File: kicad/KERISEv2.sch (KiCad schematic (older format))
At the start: 11 parts, among them SW1 RESET, U1 STM32F405RGTx

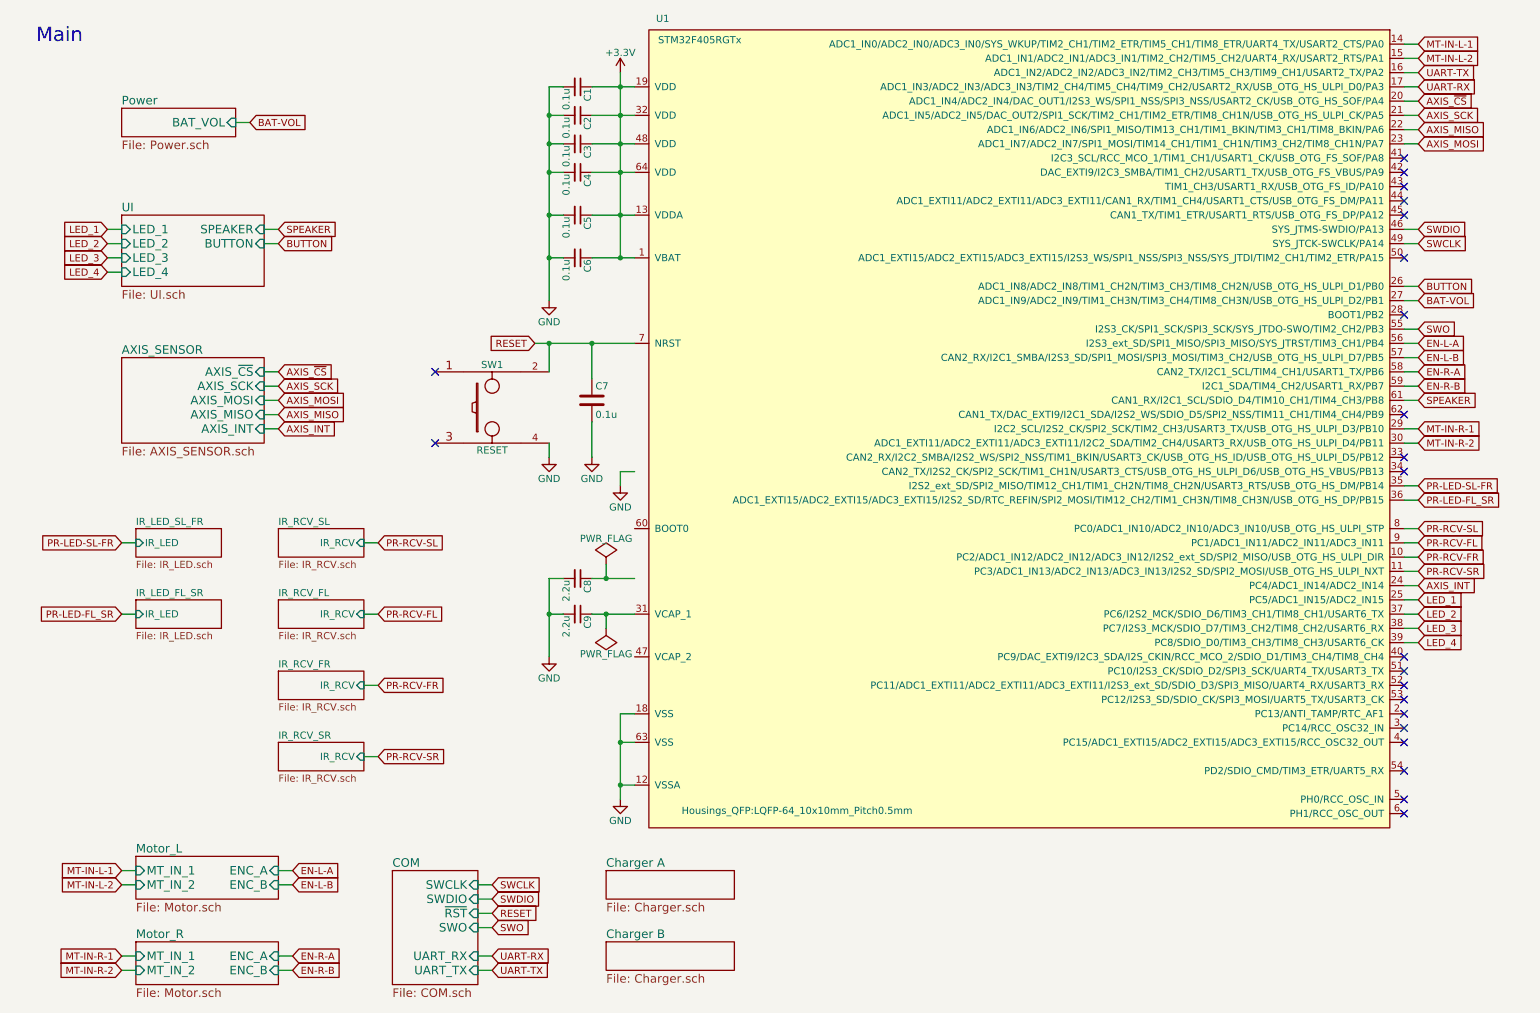
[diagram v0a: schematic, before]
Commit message: 新基板，部品を配置
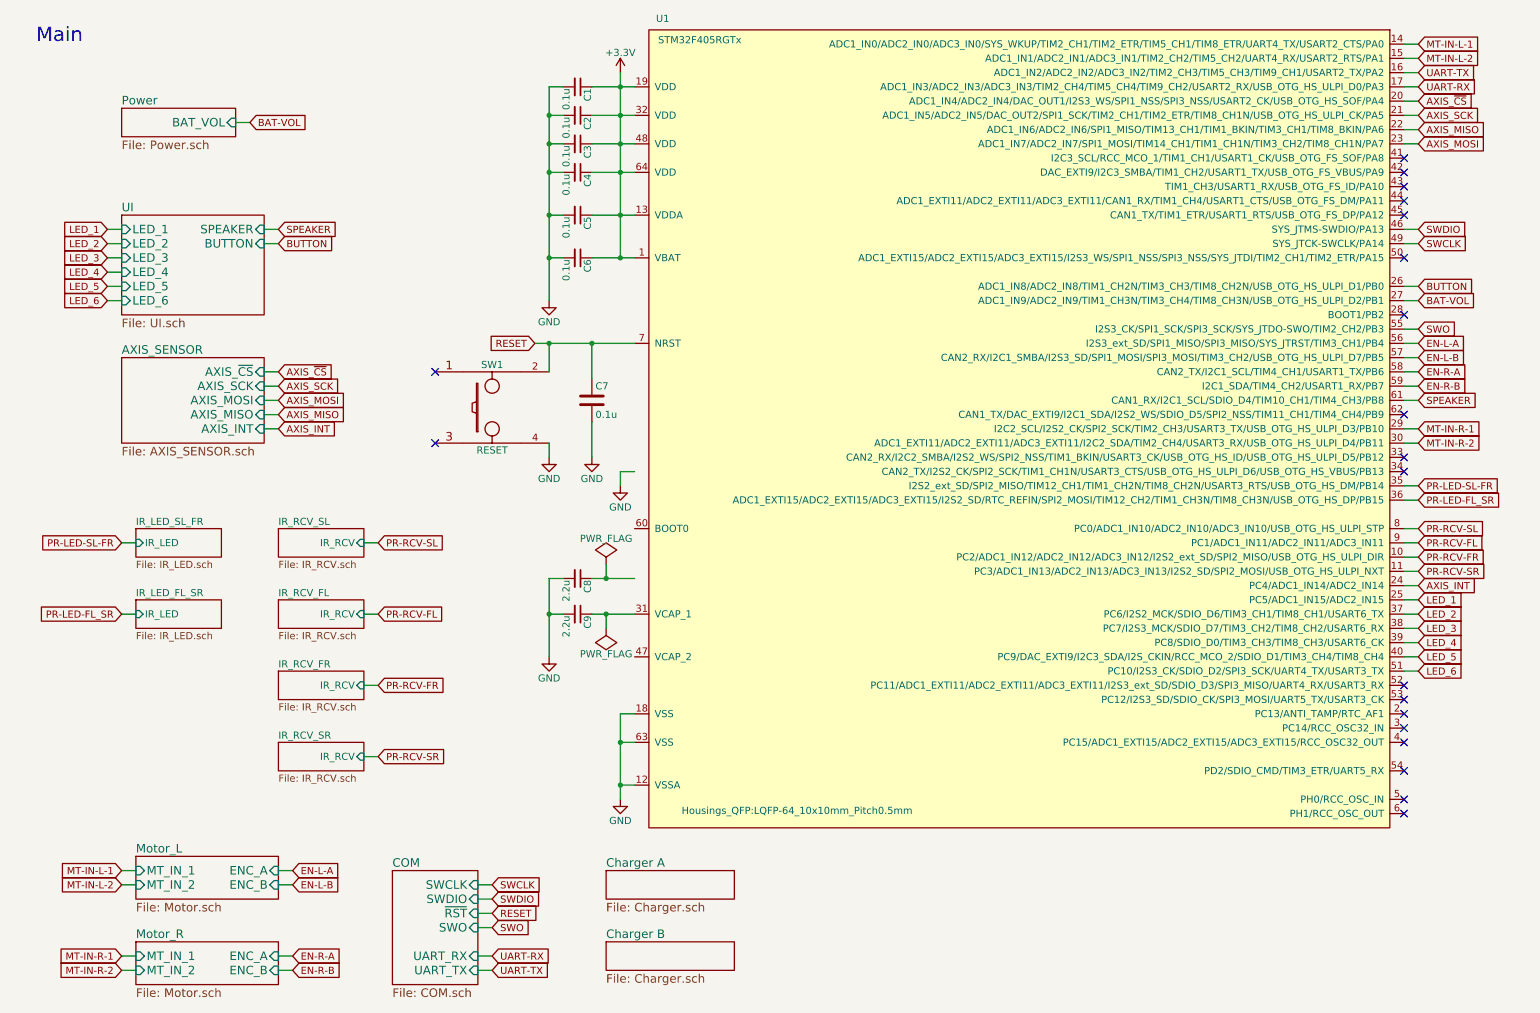
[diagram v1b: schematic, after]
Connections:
- net LED_5: now reaches U1.40 (PC9/DAC_EXTI9/I2C3_SDA/I2S_CKIN/RCC_MCO_2/SDIO_D1/TIM3_CH4/TIM8_CH4)
- net LED_6: now reaches U1.51 (PC10/I2S3_CK/SDIO_D2/SPI3_SCK/UART4_TX/USART3_TX)
- no-connect marks 22 -> 20
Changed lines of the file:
@@
 AXIS_INT
 $Sheet
-S 1300 2000 1000 500
+S 1300 2000 1000 700
 U 57CD8D81
 F0 "UI" 60
@@
 F6 "LED_4" I L 1300 2400 60
 F7 "BUTTON" I R 2300 2200 60
+F8 "LED_5" I L 1300 2500 60
+F9 "LED_6" I L 1300 2600 60
 $EndSheet
 $Sheet
@@
 NoConn ~ 10300 3700
 NoConn ~ 10300 3800
-NoConn ~ 10300 5100
-NoConn ~ 10300 5200
 NoConn ~ 10300 5300
 NoConn ~ 10300 5400
@@
 F1 "Charger.sch" 60
 $EndSheet
+Text GLabel 1200 2500 0    50   Input ~ 0
+LED_5
+Text GLabel 1200 2600 0    50   Input ~ 0
+LED_6
+Wire Wire Line
+	1200 2600 1300 2600
+Wire Wire Line
+	1300 2500 1200 2500
+Text GLabel 10400 5100 2    50   Input ~ 0
+LED_5
+Text GLabel 10400 5200 2    50   Input ~ 0
+LED_6
+Wire Wire Line
+	10400 5100 10300 5100
+Wire Wire Line
+	10300 5200 10400 5200
 $EndSCHEMATC
